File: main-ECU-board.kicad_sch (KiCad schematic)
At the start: 8 parts, among them IC1 R7FA4M1AB3CFM#AA0, J1 Power, J2 Analog, J3 Digital/PWM, J4 Digital/PWM, J5 USB_C_Receptacle

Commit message: 発注先ラベル追加
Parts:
- D1, IC1: 発注先 (none) -> Digi-Key
- D2, J5: 発注先 (none) -> 秋月電子
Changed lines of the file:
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@@
+      (effects (font (size 1.27 1.27)) hide)
+    )
+    (property "発注先" "秋月電子" (at 76.2 139.7 0)
       (effects (font (size 1.27 1.27)) hide)
     )
@@
       (effects (font (size 1.27 1.27)) hide)
     )
+    (property "発注先" "秋月電子" (at 64.77 83.82 0)
+      (effects (font (size 1.27 1.27)) hide)
+    )
     (pin "1")
     (pin "2")
@@
       (effects (font (size 1.524 1.524)) (justify left) hide)
     )
+    (property "発注先" "Digi-Key" (at 39.37 181.61 0)
+      (effects (font (size 1.27 1.27)) hide)
+    )
     (pin "1")
     (pin "2")
@@
       (effects (font (size 1.27 1.27)) (justify left) hide)
     )
-    (pin "1")
+    (property "発注先" "Digi-Key" (at 101.6 63.5 0)
+      (effects (font (size 1.27 1.27)) hide)
+    )
+    (pin "1")

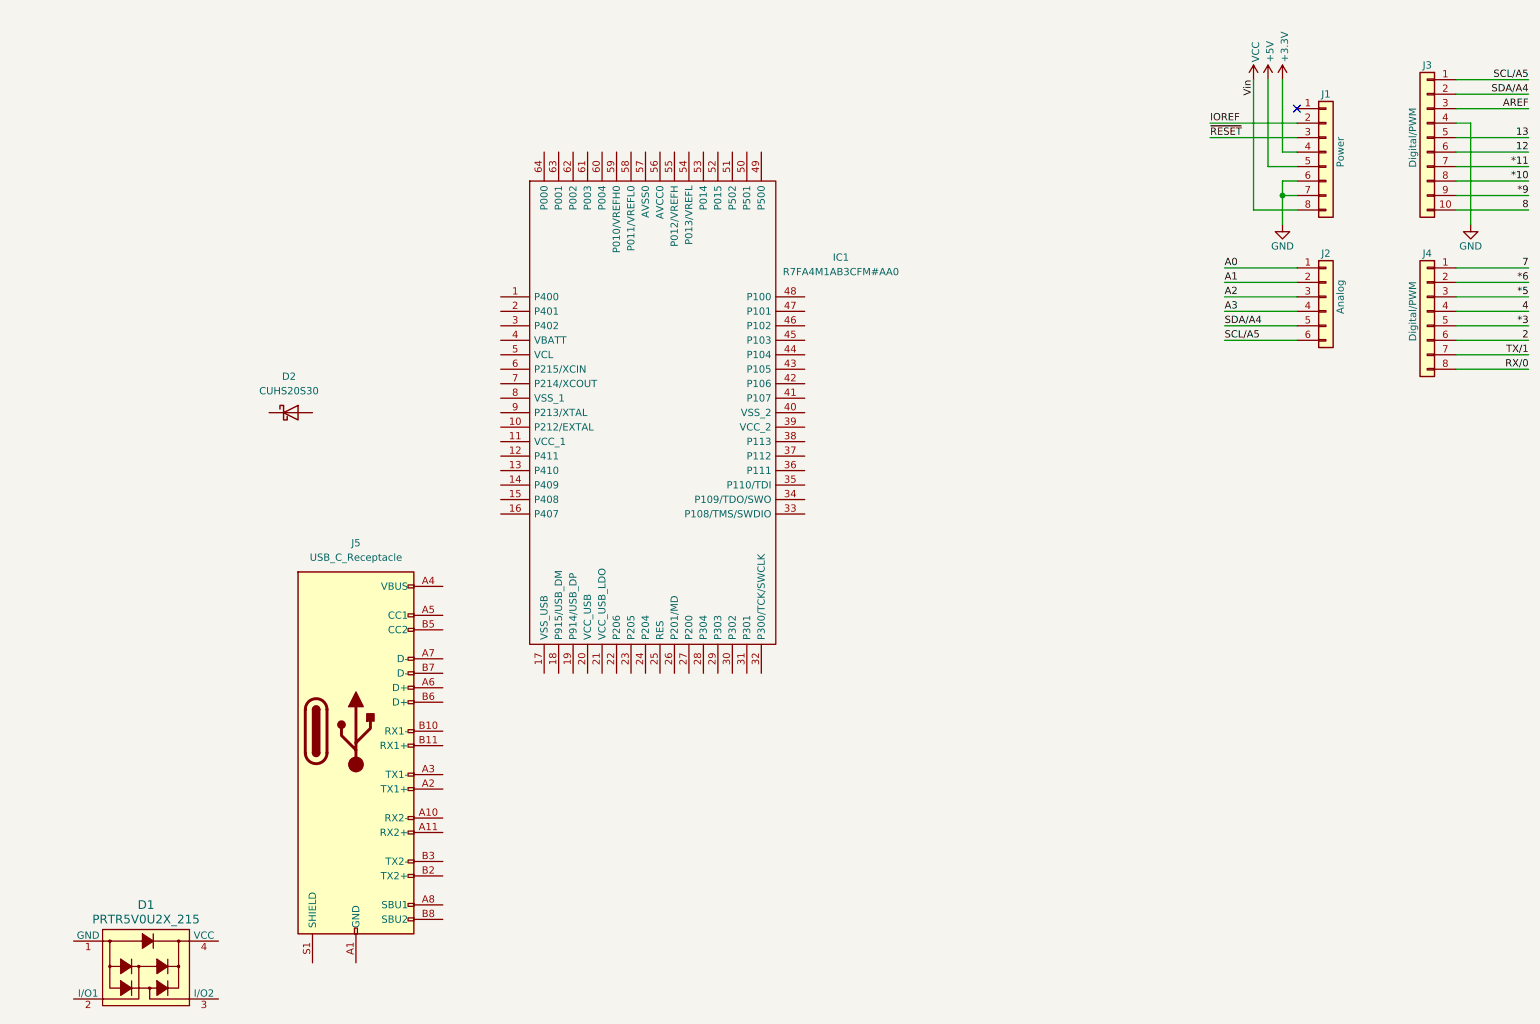
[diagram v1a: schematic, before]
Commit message: usb周り修正
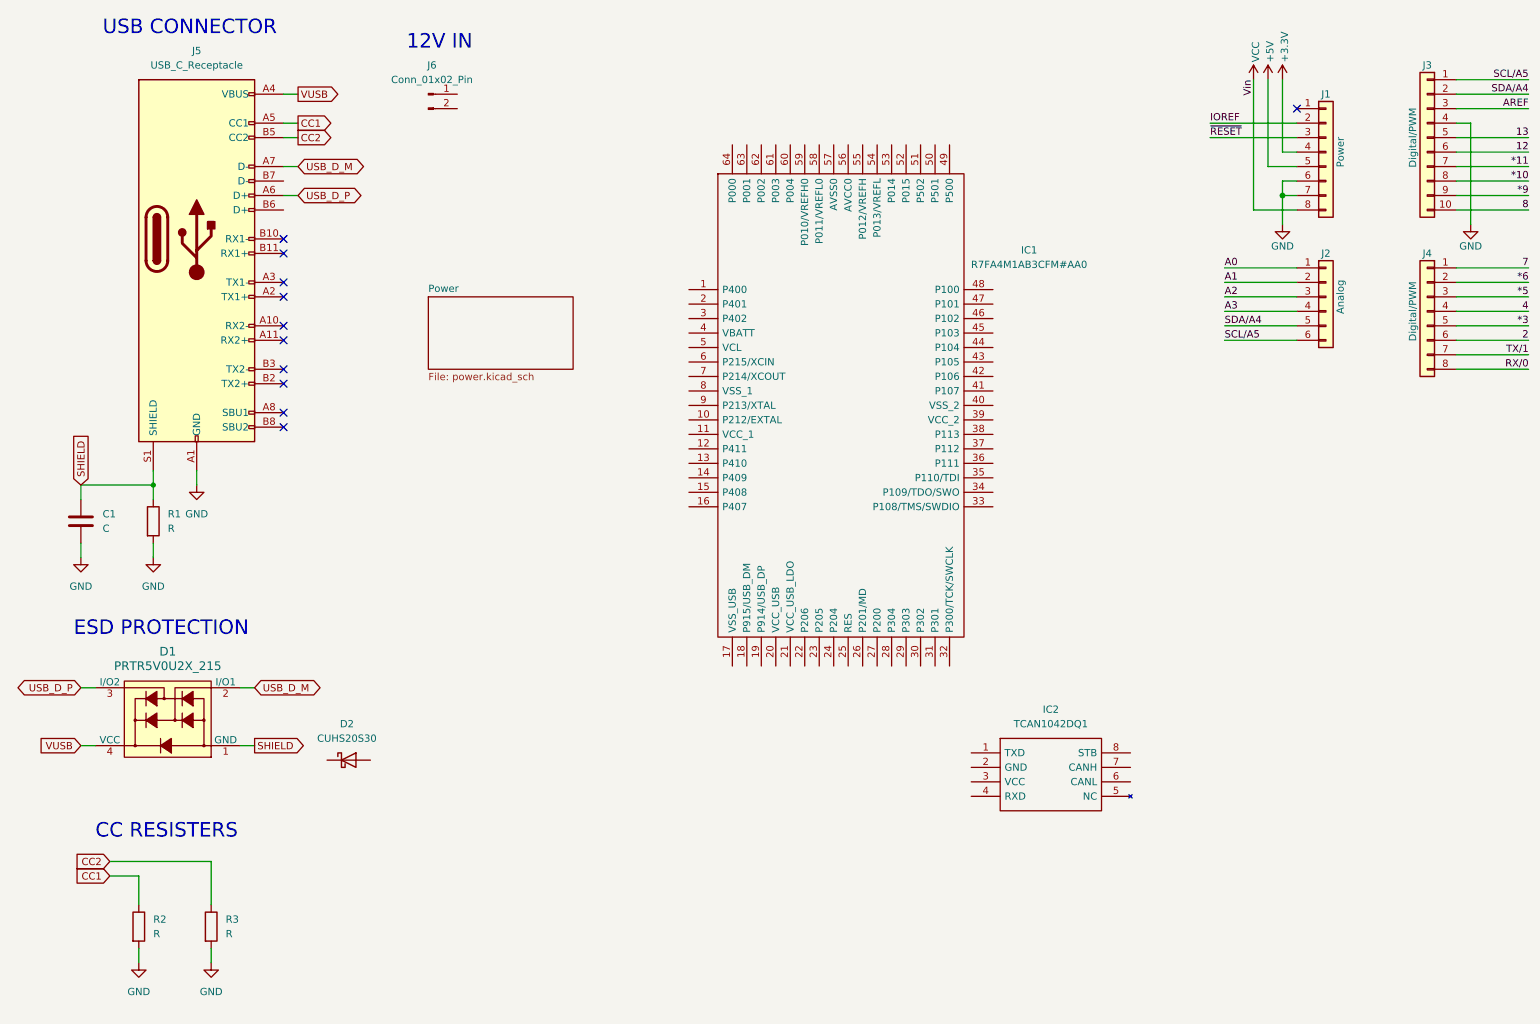
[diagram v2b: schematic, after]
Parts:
- added C1: C, symbol Device:C
- added IC2: TCAN1042DQ1, SOIC127P600X175-8N, symbol SamacSys_Parts:TCAN1042DQ1
- added J6: Conn_01x02_Pin, symbol Connector:Conn_01x02_Pin
- added R1, R2, R3: R, symbol Device:R
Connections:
- net GND: now also J5.A1 (GND), J5.A12 (GND), J5.B1 (GND), J5.B12 (GND), C1.2, R1.2, R2.2, R3.2
- net VUSB: now reaches J5.A4 (VBUS), J5.A9 (VBUS), J5.B4 (VBUS), J5.B9 (VBUS)
- net VUSB: now also D1.4 (VCC)
- net CC1: now reaches J5.A5 (CC1)
- net CC1: now also R2.1
- net USB_D_P: now reaches J5.A6 (D+)
- net USB_D_P: now also D1.3 (I/O2)
- net USB_D_M: now reaches J5.A7 (D-)
- net USB_D_M: now also D1.2 (I/O1)
- net CC2: now reaches J5.B5 (CC2)
- net CC2: now also R3.1
- net SHIELD: now reaches J5.S1 (SHIELD)
- net SHIELD: now also D1.1 (GND), C1.1, R1.1
- no-connect marks 1 -> 11
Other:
- added sheet Power (power.kicad_sch)
- note added: "12V IN"
- note added: "CC RESISTERS"
- note added: "ESD PROTECTION"
- note added: "USB CONNECTOR"
- moved on the sheet: D1, D2, IC1, J5
